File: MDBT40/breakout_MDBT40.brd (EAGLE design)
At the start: 30.5 x 72.9 mm, 18 parts

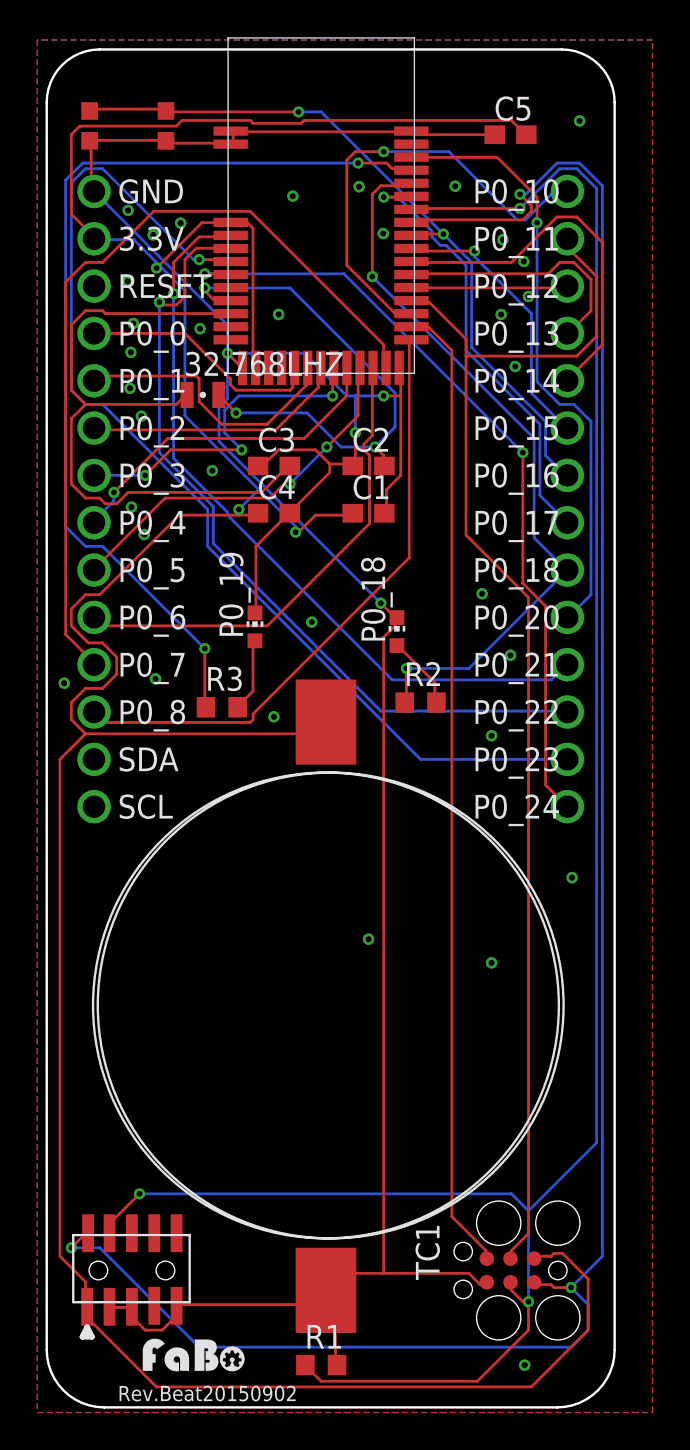
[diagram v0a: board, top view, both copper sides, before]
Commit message: Add update
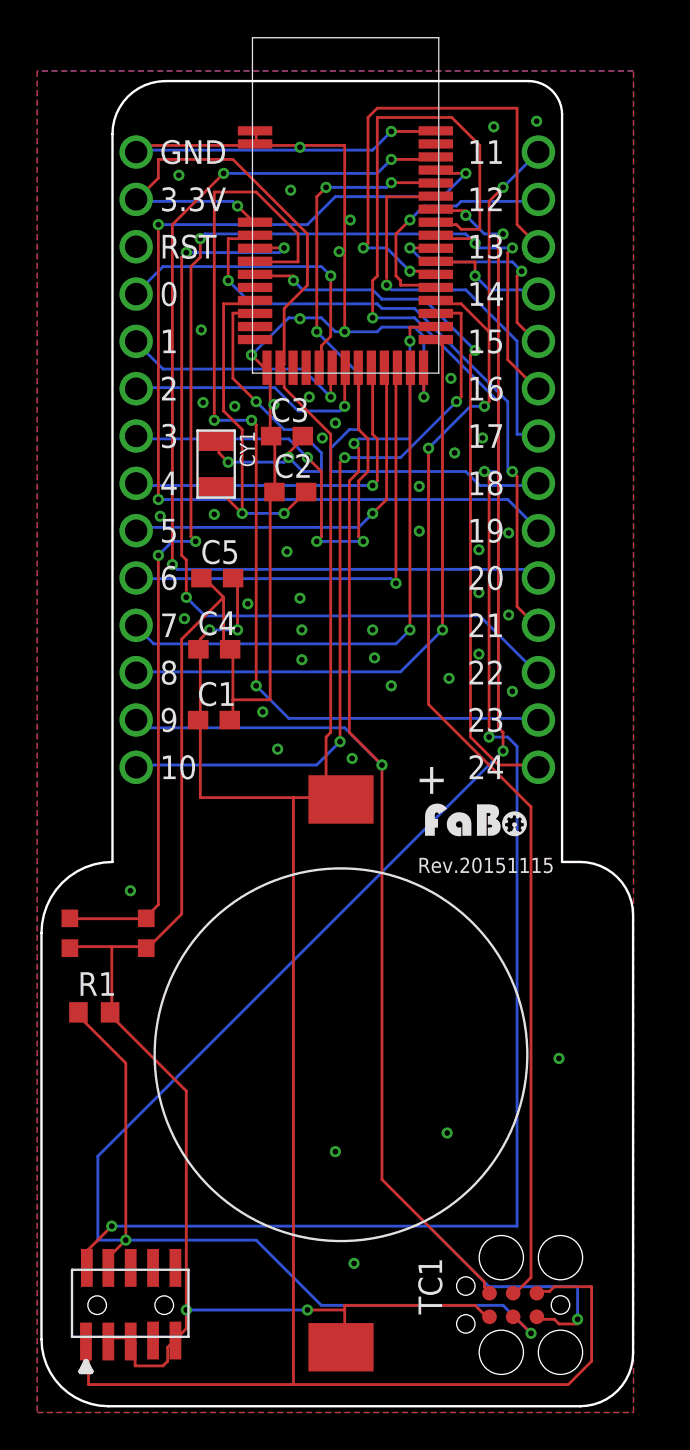
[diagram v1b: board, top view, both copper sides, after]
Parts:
- removed 32.768LHZ: FC-12M, crystal:FC-12M
- removed P0_18, P0_19: (no value), led:CHIP-LED0603
- removed R2, R3: (no value), adafruit:R0603
- removed U$2: SMTU2450-TOP, GClue-Supply:SMTU2450
- added CY1: (no value), FaBo-Crystal:ABRACOM-ABS07-32.768KHZ
- added U$8: SMTU-TOP2032, FaBo-Supply:SMTU-2032
- U$3: value BREAKOUT_BLE_NORDIC -> BLE-BREAKOUT-NORDIC; device gclue:BREAKOUT_BLE_NORDIC -> FaBo-Template:BLE-BREAKOUT-NORDIC
- moved U$5 43.3 mm to (2.75, 26.5)
- moved U$7 32.5 mm to (23.6, 30.9)
- moved C5 28.5 mm to (9.66, 44.8)
- moved R1 22.5 mm to (3.06, 21.5)
- moved C1 13.9 mm to (9.48, 37.2)
- moved C4 7.97 mm to (9.50, 41.0)
- moved C2 4.43 mm to (13.6, 49.4)
- moved U$3 4.35 mm to (16.7, 34.6)
- moved U$4 1.86 mm to (5.01, 5.76)
- moved TC1 1.86 mm to (25.5, 5.77)
- moved C3 1.75 mm to (13.4, 52.4)
- moved U$1 1.31 mm to (16.5, 64.8)
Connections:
- removed net N$1: P0_18.A, R2.2
- removed net N$2: P0_19.A, R3.2
- net +3V3: now also U$8.+; no longer U$2.P$_VCC
- net GND: now also U$8.-; no longer P0_18.C, P0_19.C, U$2.P$_GND
- net N$7: now also CY1.P$2; no longer 32.768LHZ.2
- net N$8: now also CY1.P$1; no longer 32.768LHZ.1
- net P0_00: now also U$3.0; no longer U$3.P0_0
- net P0_01: now also U$3.1; no longer U$3.P0_1
- net P0_02: now also U$3.2; no longer U$3.P0_2
- net P0_03: now also U$3.3; no longer U$3.P0_3
- net P0_04: now also U$3.4; no longer U$3.P0_4
- net P0_05: now also U$3.5; no longer U$3.P0_5
- net P0_06: now also U$3.6; no longer U$3.P0_6
- net P0_07: now also U$3.7; no longer U$3.P0_7
- net P0_08: now also U$3.8; no longer U$3.P0_8
- net P0_09: now also U$3.9
- net P0_10: now also U$3.10; no longer U$3.P1_0
- net P0_11: now also U$3.11; no longer U$3.P1_1
- net P0_12: now also U$3.12; no longer U$3.P1_2
- net P0_13: now also U$3.13; no longer U$3.P1_3
- net P0_14: now also U$3.14; no longer U$3.P1_4
- net P0_15: now also U$3.15; no longer U$3.P1_5
- net P0_16: now also U$3.16; no longer U$3.P1_6
- net P0_17: now also U$3.17; no longer U$3.P1_7
- net P0_18: now also U$3.18; no longer R2.1, U$3.P1_8
- net P0_19: now also U$3.19; no longer R3.1
- net P0_20: now also U$3.20; no longer U$3.P2_0
- net P0_21: now also U$3.21; no longer U$3.P2_1
- net P0_22: now also U$3.22; no longer U$3.P2_2
- net P0_23: now also U$3.23; no longer U$3.P2_3
- net P0_24: now also U$3.24; no longer U$3.P2_4
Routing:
- net +3V3: track 176.2 -> 142.1 mm
- net P0_16: track 39.3 -> 70.7 mm, vias 2 -> 5
- net P0_09: track 52.2 -> 73.7 mm, vias 0 -> 3
- net P0_20: track 32.4 -> 53.9 mm, vias 1 -> 3
- net N$8: track 36.7 -> 20.4 mm, vias 0 -> 3
- net P0_10: track 24.4 -> 40.3 mm, vias 1 -> 3
- net P0_07: track 44.1 -> 29.5 mm, vias 0 -> 1
- net P0_13: track 13.7 -> 27.7 mm, vias 0 -> 2
- net P0_14: track 20.0 -> 6.69 mm, vias 0 -> 1
- net N$7: track 28.5 -> 19.3 mm, vias 3 -> 2
- net P0_03: track 18.6 -> 26.9 mm
- net SWDIO: track 109.7 -> 117.1 mm, vias 3 -> 5
- net P0_21: track 40.7 -> 34.4 mm, vias 1 -> 2
- net P0_18: track 39.6 -> 34.8 mm, vias 2 -> 3
- net P0_12: track 8.41 -> 13.2 mm, vias 0 -> 1
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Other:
- board size 30.5 x 72.9 mm -> 31.8 x 71.1 mm
- board text added: "Rev.20151115"
- board text removed: "Rev.Beat20150902"
